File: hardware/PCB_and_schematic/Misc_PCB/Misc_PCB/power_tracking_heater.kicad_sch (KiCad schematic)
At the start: 9 parts, among them J6 PROG_INTERFACE, Q13 BC817, Q14 BC817, U9 ESP-07

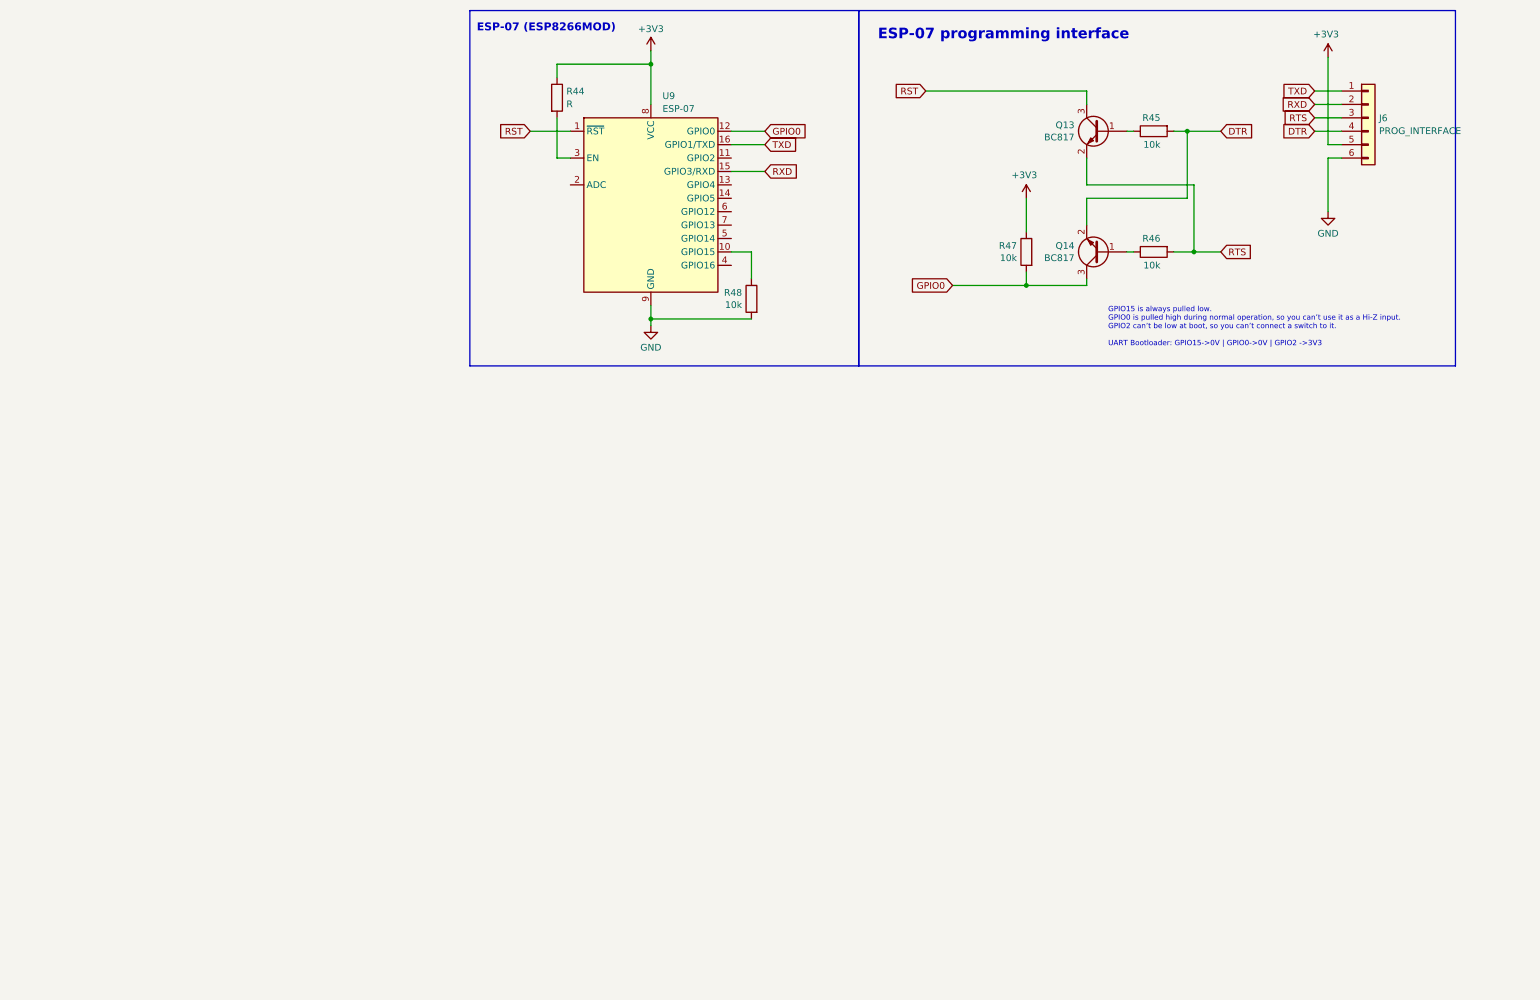
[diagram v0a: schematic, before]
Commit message: progress with esp power pcb
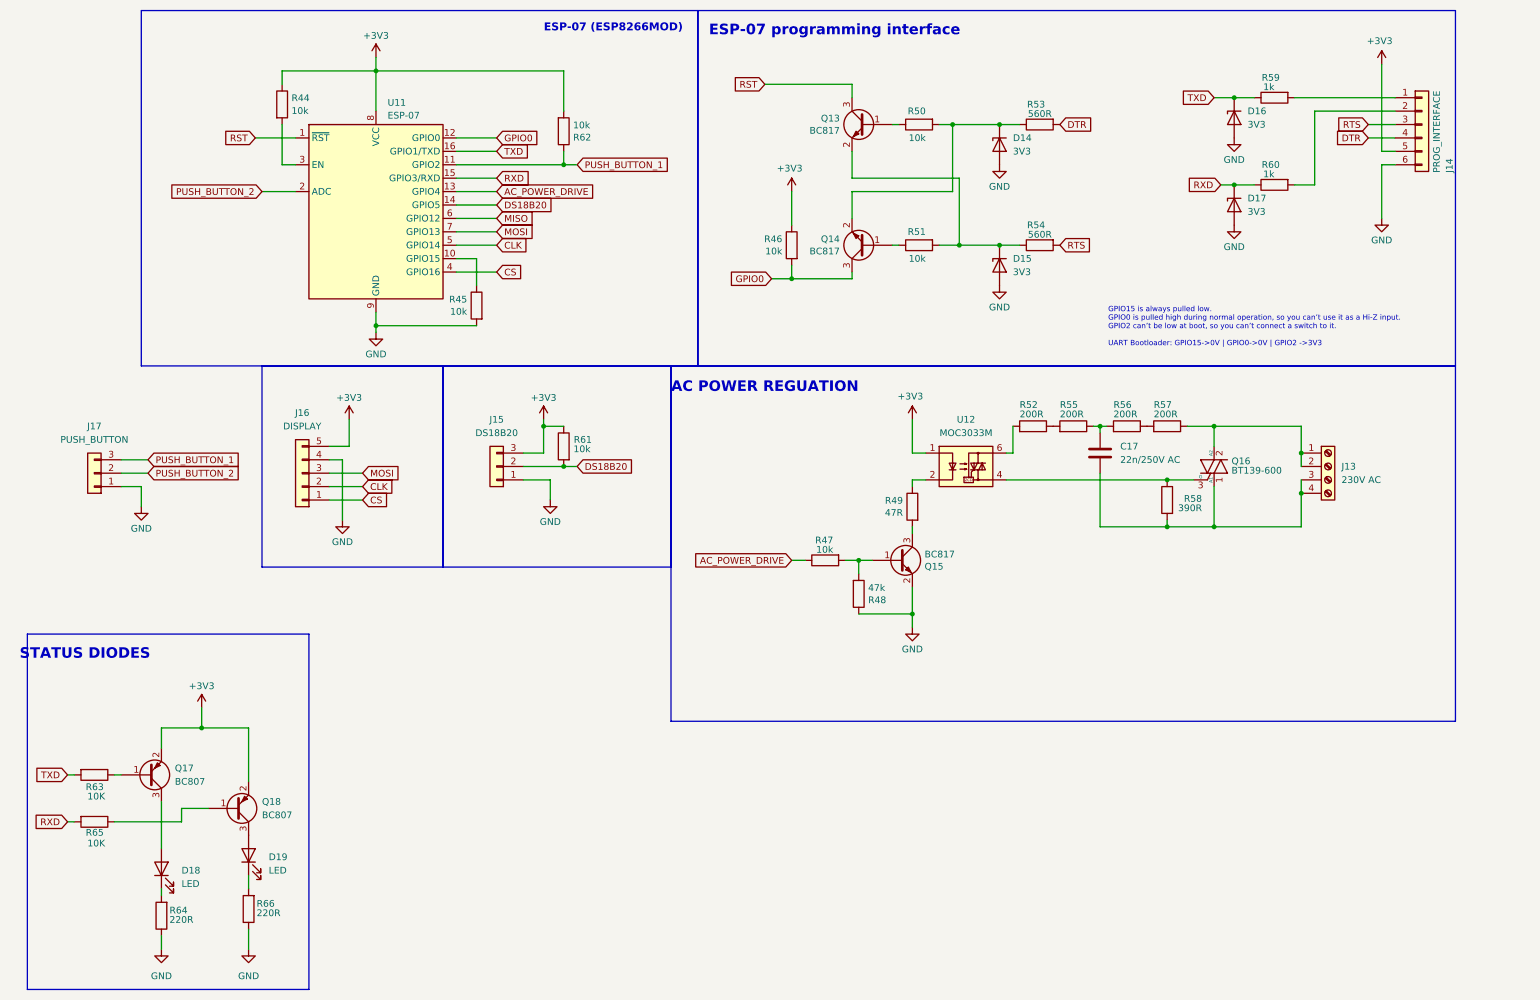
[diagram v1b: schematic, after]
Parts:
- added C17: 22n/250V AC, symbol Device:C
- added D14, D15, D16, D17: 3V3, symbol Device:D_Zener
- added D18, D19: LED, LED_SMD:LED_PLCC-2_3.4x3.0mm_KA, symbol Device:LED
- added J13: 230V AC, symbol Connector:Screw_Terminal_01x04
- added J15: DS18B20, symbol Connector_Generic:Conn_01x03
- added J16: DISPLAY, symbol Connector_Generic:Conn_01x05
- added J17: PUSH_BUTTON, symbol Connector_Generic:Conn_01x03
- added Q15: BC817, TO_SOT_Packages_SMD:SOT-23_Handsoldering, symbol Transistor_BJT:BC817
- added Q16: BT139-600, Package_TO_SOT_THT:TO-220-3_Vertical, symbol Triac_Thyristor:BT139-600
- added Q17, Q18: BC807, Package_TO_SOT_SMD:SOT-23, symbol Transistor_BJT:BC807
- added R47, R61, R62: 10k, Resistors_SMD:R_0805_HandSoldering, symbol Device:R
- added R48: 47k, Resistors_SMD:R_0805_HandSoldering, symbol Device:R
- added R49: 47R, Resistors_SMD:R_0805_HandSoldering, symbol Device:R
- added R52, R55, R56, R57: 200R, Resistor_THT:R_Axial_DIN0204_L3.6mm_D1.6mm_P7.62mm_Horizontal, symbol Device:R
- added R53, R54: 560R, Resistors_SMD:R_0805_HandSoldering, symbol Device:R
- added R58: 390R, Resistor_THT:R_Axial_DIN0204_L3.6mm_D1.6mm_P7.62mm_Horizontal, symbol Device:R
- added R59, R60: 1k, Resistors_SMD:R_0805_HandSoldering, symbol Device:R
- added R63, R65: 10K, Resistor_SMD:R_0805_2012Metric_Pad1.20x1.40mm_HandSolder, symbol Device:R
- added R64, R66: 220R, Resistor_SMD:R_0805_2012Metric_Pad1.20x1.40mm_HandSolder, symbol Device:R
- added U12: MOC3033M, symbol Relay_SolidState:MOC3033M
- R44: value R -> 10k
- renumbered J6 to J14, R48 to R45, R47 to R46, R45 to R50, R46 to R51, U9 to U11
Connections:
- net +3V3: now also J15.3 (Pin_3), J16.5 (Pin_5), Q17.2 (E), Q18.2 (E), R61.1, R62.2, U12.1
- net DTR: now also R53.2; no longer Q14.2 (E), R50.2
- net GND: now also D14.2 (A), D15.2 (A), D16.2 (A), D17.2 (A), J15.1 (Pin_1), J16.4 (Pin_4), J17.1 (Pin_1), Q15.2 (E), R48.1, R64.1, R66.1
- net RTS: now also R54.2; no longer Q13.2 (E), R51.2
- net RXD: now also D17.1 (K), R60.1, R65.2; no longer J14.2 (Pin_2)
- net TXD: now also D16.1 (K), R59.1, R63.2; no longer J14.1 (Pin_1)
- net PUSH_BUTTON_1: now reaches U11.11 (GPIO2)
- net PUSH_BUTTON_1: now also J17.3 (Pin_3), R62.1
- net AC_POWER_DRIVE: now reaches U11.13 (GPIO4)
- net AC_POWER_DRIVE: now also R47.1
- net DS18B20: now reaches U11.14 (GPIO5)
- net DS18B20: now also J15.2 (Pin_2), R61.2
- net PUSH_BUTTON_2: now reaches U11.2 (ADC)
- net PUSH_BUTTON_2: now also J17.2 (Pin_2)
- net CS: now reaches U11.4 (GPIO16)
- net CS: now also J16.1 (Pin_1)
- net CLK: now reaches U11.5 (GPIO14)
- net CLK: now also J16.2 (Pin_2)
- net MISO: now reaches U11.6 (GPIO12)
- net MOSI: now reaches U11.7 (GPIO13)
- net MOSI: now also J16.3 (Pin_3)
- new net: Q16.3 (G), R58.1, U12.4
- new net: C17.2, J13.3 (Pin_3), J13.4 (Pin_4), Q16.1 (A1), R58.2
- new net: Q17.1 (B), R63.1
- new net: C17.1, R55.1, R56.2
- new net: R52.1, R55.2
- new net: D14.1 (K), Q14.2 (E), R50.2, R53.1
- new net: R49.1, U12.2
- new net: R52.2, U12.6
- new net: Q18.1 (B), R65.1
- new net: D19.2 (A), Q18.3 (C)
- new net: J13.1 (Pin_1), J13.2 (Pin_2), Q16.2 (A2), R57.1
- new net: D18.2 (A), Q17.3 (C)
- new net: D15.1 (K), Q13.2 (E), R51.2, R54.1
- new net: D19.1 (K), R66.2
- new net: Q15.1 (B), R47.2, R48.2
- new net: Q15.3 (C), R49.2
- new net: J14.1 (Pin_1), R59.2
- new net: J14.2 (Pin_2), R60.2
- new net: D18.1 (K), R64.2
- new net: R56.1, R57.2
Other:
- note added: "AC POWER REGUATION"
- note added: "STATUS DIODES"
- moved on the sheet: J14, Q13, Q14, R44, R45, R46, R50, R51, U11
